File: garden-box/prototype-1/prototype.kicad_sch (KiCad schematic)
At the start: 16 parts, among them J1 Conn_01x05_Male, J2 Screw_Terminal_01x02, Q1 IRF830, U1 4N35

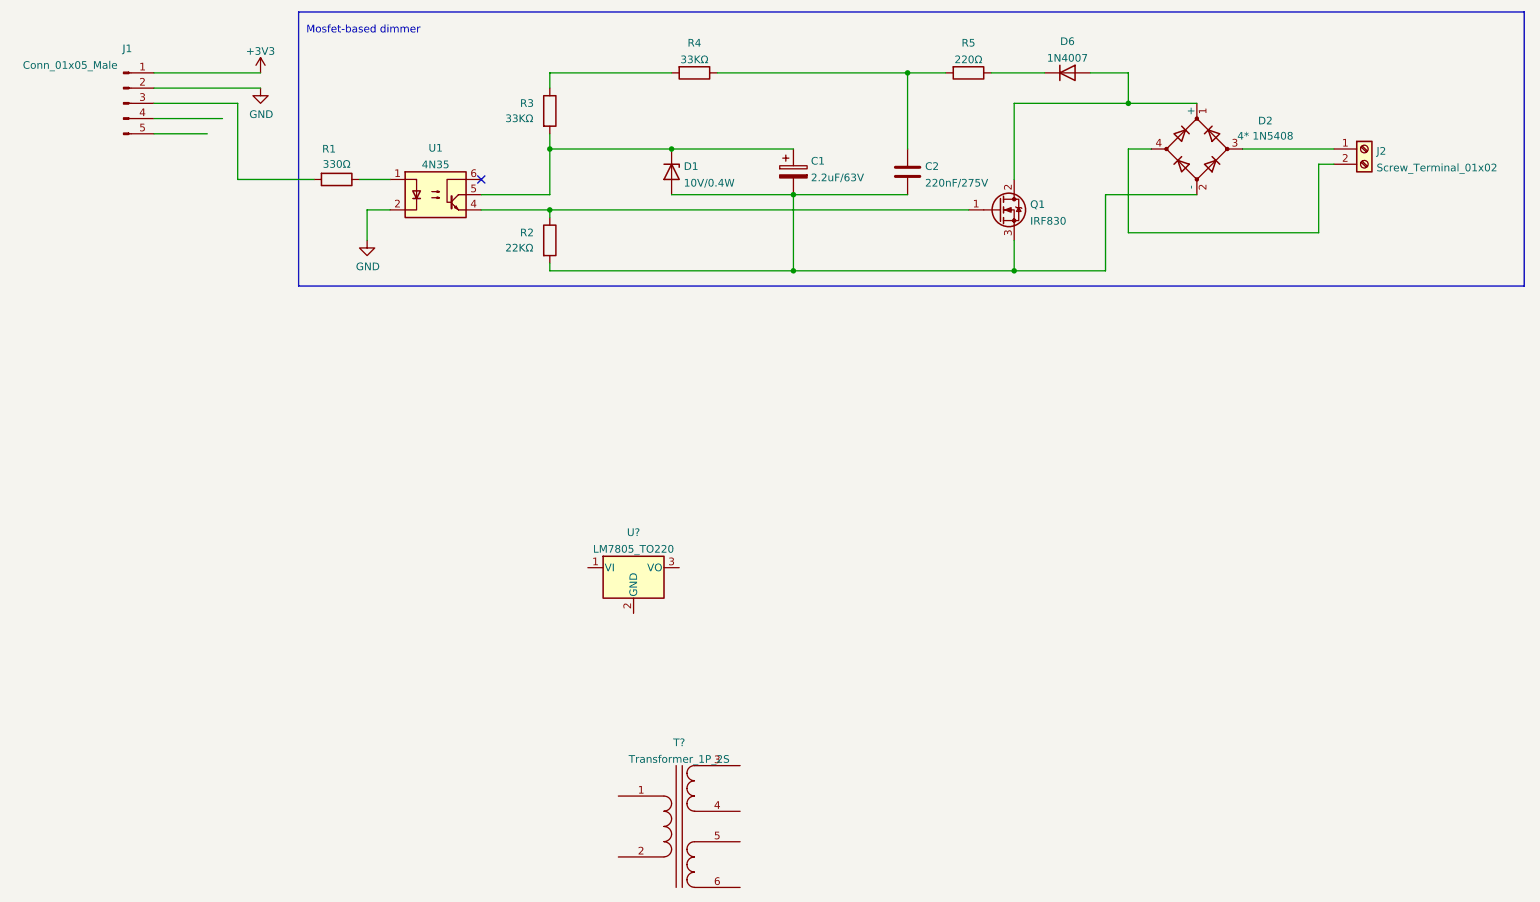
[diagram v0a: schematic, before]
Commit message: wip garden box
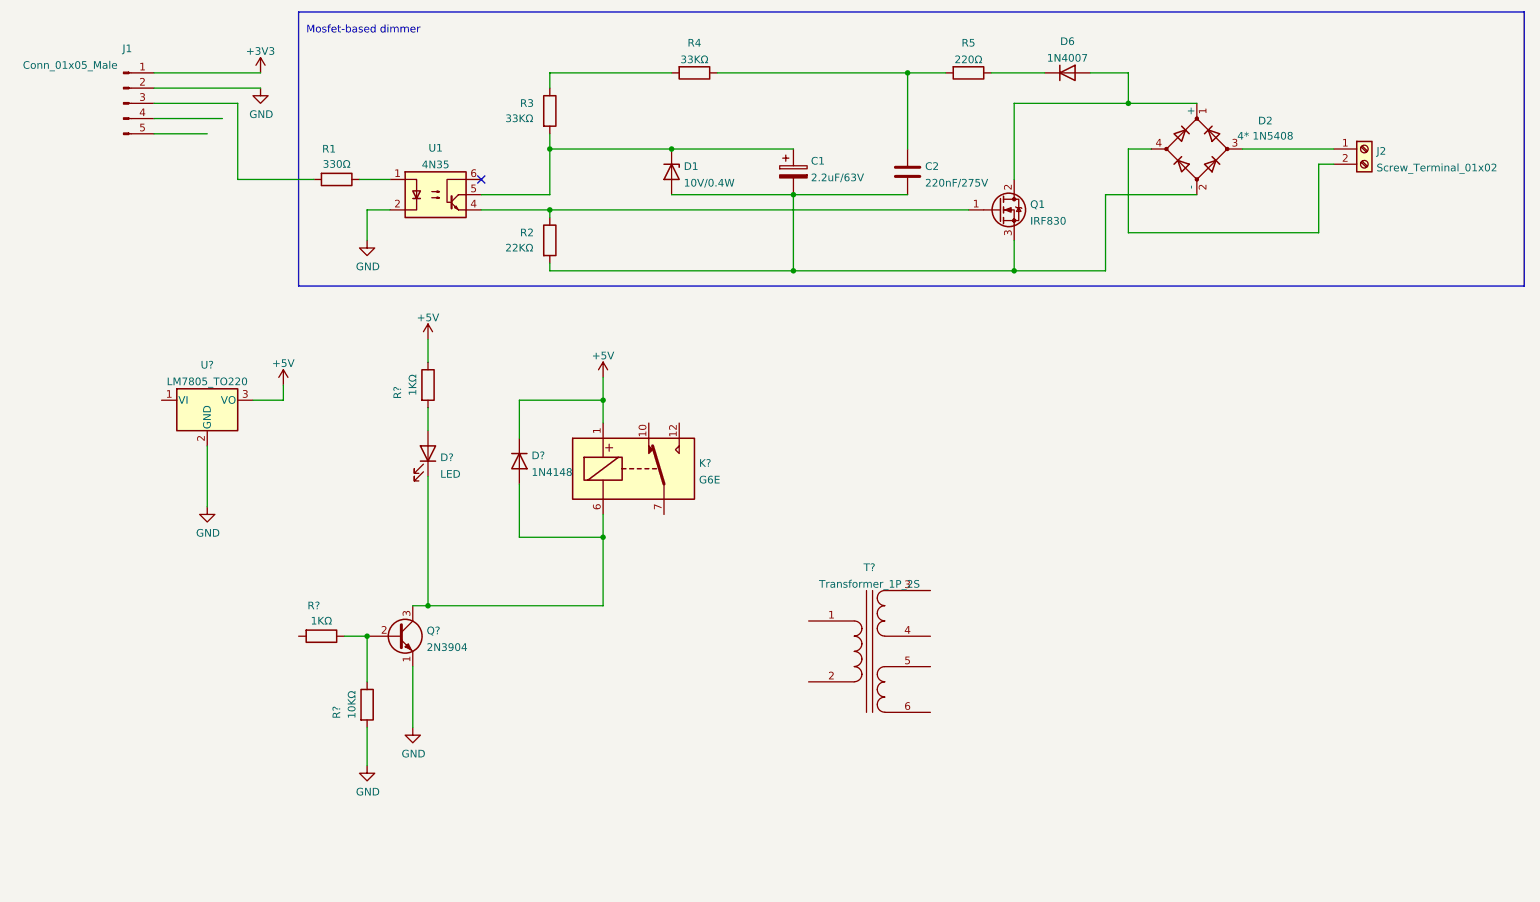
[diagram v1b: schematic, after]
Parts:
- added D?: LED, symbol Device:LED
- added D?: 1N4148, Diode_THT:D_DO-35_SOD27_P7.62mm_Horizontal, symbol Diode:1N4148
- added K?: G6E, Relay_THT:Relay_SPDT_Omron_G6E, symbol Relay:G6E
- added Q?: 2N3904, Package_TO_SOT_THT:TO-92_Inline, symbol Transistor_BJT:2N3904
- added R? (x2): 1KΩ, Resistor_SMD:R_0603_1608Metric, symbol Device:R
- added R?: 10KΩ, Resistor_SMD:R_0603_1608Metric, symbol Device:R
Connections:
- net GND: now also U?.2 (GND), Q?.1 (E), R?.2
- net +5V: now reaches U?.3 (VO)
- net +5V: now also D?.1 (K), K?.1, R?.1
- new net: D?.1 (K), D?.2 (A), K?.6, Q?.3 (C)
- new net: D?.2 (A), R?.2
- new net: Q?.2 (B), R?.1, R?.1
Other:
- moved on the sheet: T?, U?
